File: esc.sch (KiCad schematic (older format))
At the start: 65 parts, among them IC1 4N25, IC2 LM25101, IC3 LM25101, IC4 LM25101, IC5 ATMEGA8-AI, P1 CONN_01X03, P2 CONN_01X03, P3 CONN_01X02, P4 CONN_02X02, Q1 MOSFET_N, Q10 MOSFET_N, Q11 MOSFET_N, Q12 MOSFET_N, Q2 MOSFET_N, Q3 MOSFET_N, Q4 MOSFET_N, Q5 MOSFET_N, Q6 MOSFET_N, Q7 MOSFET_N, Q8 MOSFET_N, Q9 MOSFET_N, U1 MCP1804, U2 LM2940 10V, Y1 RESONATEUR

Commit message: PCB almost done!
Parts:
- C10, C12, C13, C14, C15, C16, C17, C18, C4, C5, C7: symbol C -> C-RESCUE-esc
- IC1: symbol 4N25 -> 4N25-RESCUE-esc
- R1, R10, R11, R12, R13, R14, R15, R17, R18, R19, R2, R20, R21, R22, R3, R4, R5, R6, R8, R9: symbol R -> R-RESCUE-esc
- R16, R7: footprint Resistors_SMD:R_0805_HandSoldering -> Resistors_SMD:R_0603_HandSoldering; symbol R -> R-RESCUE-esc

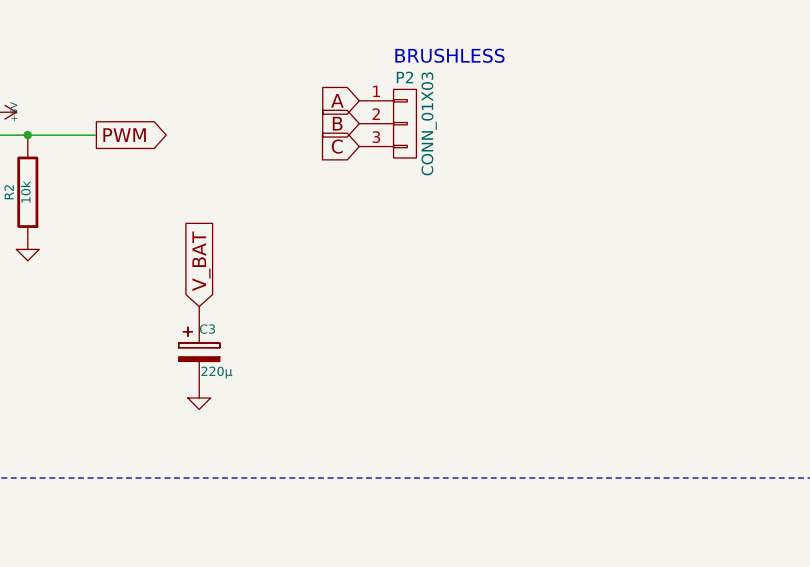
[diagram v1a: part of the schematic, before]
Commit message: PCB V1.0
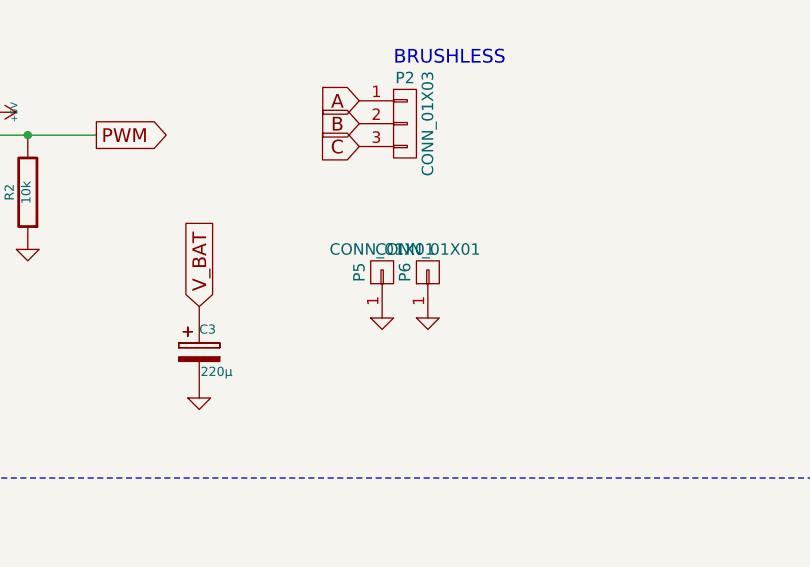
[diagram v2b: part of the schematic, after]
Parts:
- added P5, P6: CONN_01X01, Connect:1pin, symbol CONN_01X01
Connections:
- net GND: now also P5.1 (P1), P6.1 (P1)
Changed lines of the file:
@@
 Wire Wire Line
 	13200 2300 13200 2500
+$Comp
+L CONN_01X01 P5
+U 1 1 564C4523
+P 4500 1900
+F 0 "P5" H 4500 2000 50  0000 C CNN
+F 1 "CONN_01X01" V 4600 1900 50  0000 C CNN
+F 2 "Connect:1pin" H 4500 1900 60  0001 C CNN
+F 3 "" H 4500 1900 60  0000 C CNN
+	1    4500 1900
+	0    -1   -1   0
+$EndComp
+$Comp
+L CONN_01X01 P6
+U 1 1 564C47FE
+P 4700 1900
+F 0 "P6" H 4700 2000 50  0000 C CNN
+F 1 "CONN_01X01" V 4800 1900 50  0000 C CNN
+F 2 "Connect:1pin" H 4700 1900 60  0001 C CNN
+F 3 "" H 4700 1900 60  0000 C CNN
+	1    4700 1900
+	0    -1   -1   0
+$EndComp
+$Comp
+L GND-RESCUE-esc #PWR047
+U 1 1 564C48DB
+P 4500 2100
+F 0 "#PWR047" H 4500 2100 30  0001 C CNN
+F 1 "GND" H 4500 2030 30  0001 C CNN
+F 2 "" H 4500 2100 60  0000 C CNN
+F 3 "" H 4500 2100 60  0000 C CNN
+	1    4500 2100
+	1    0    0    -1
+$EndComp
+$Comp
+L GND-RESCUE-esc #PWR048
+U 1 1 564C49AF
+P 4700 2100
+F 0 "#PWR048" H 4700 2100 30  0001 C CNN
+F 1 "GND" H 4700 2030 30  0001 C CNN
+F 2 "" H 4700 2100 60  0000 C CNN
+F 3 "" H 4700 2100 60  0000 C CNN
+	1    4700 2100
+	1    0    0    -1
+$EndComp
 $EndSCHEMATC
